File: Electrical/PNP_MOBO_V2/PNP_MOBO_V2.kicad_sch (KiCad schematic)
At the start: 48 parts, among them J1 USB_C_Receptacle_USB2.0_16P, J4 Conn_01x03_Pin, J6 Conn_01x03_Pin, J8 Barrel_Jack_MountingPin, SW1 SW_Push, SW2 SW_Push, U1 ESP32-S3-WROOM-1, U3 SN65HVD230, U4 AMS1117-3.3

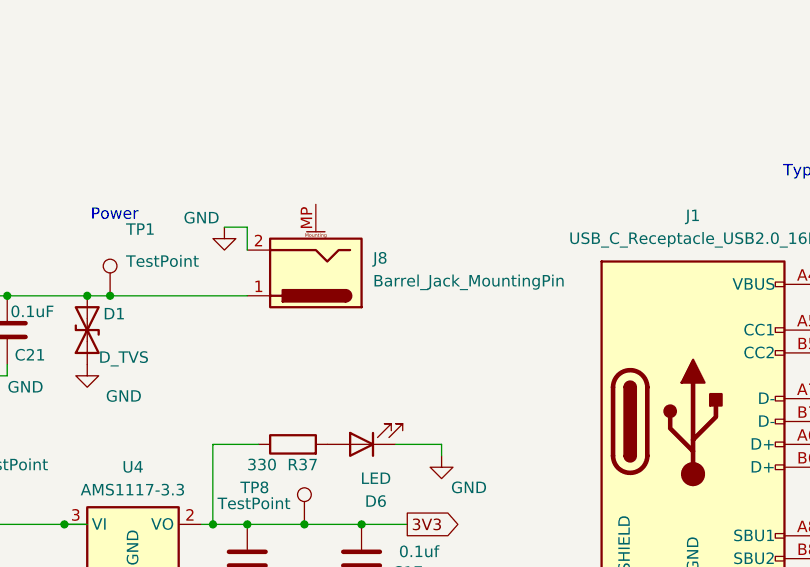
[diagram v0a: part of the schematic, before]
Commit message: fix: last change before order
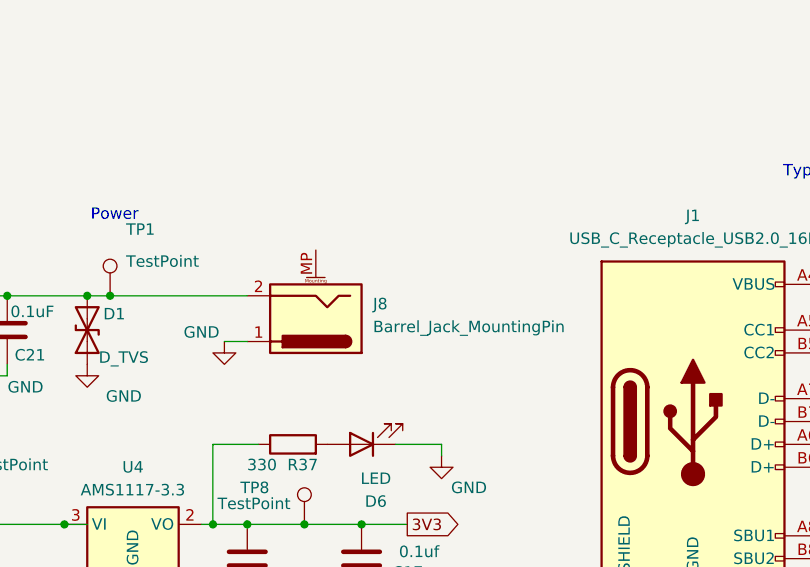
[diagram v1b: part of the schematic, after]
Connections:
- net 12V: now also J8.2; no longer J8.1
- net GND: now also J8.1; no longer J8.2
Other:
- moved on the sheet: J8
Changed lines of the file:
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@@
 	)
 	(junction
+		(at 39.37 151.13)
+		(diameter 0)
+		(color 0 0 0 0)
+	)
+	(junction
 		(at 60.96 184.15)
 		(diameter 0)
@@
 	)
 	(junction
-		(at 39.37 151.13)
-		(diameter 0)
-		(color 0 0 0 0)
-	)
-	(junction
 		(at 229.87 41.91)
 		(diameter 0)
@@
 	(wire
 		(pts
-			(xy 54.61 143.51) (xy 52.07 143.51)
+			(xy 54.61 156.21) (xy 52.07 156.21)
 		)
 		(stroke
@@
 	(wire
 		(pts
-			(xy 39.37 151.13) (xy 54.61 151.13)
-		)
-		(stroke
-			(width 0)
-			(type default)
-		)
-	)
-	(wire
-		(pts
 			(xy 27.94 160.02) (xy 25.4 160.02)
 		)
@@
 	(wire
 		(pts
-			(xy 54.61 146.05) (xy 54.61 143.51)
-		)
-		(stroke
-			(width 0)
-			(type default)
-		)
-	)
-	(wire
-		(pts
 			(xy 229.87 20.32) (xy 229.87 29.21)
 		)
@@
 	(wire
 		(pts
+			(xy 39.37 151.13) (xy 54.61 151.13)
+		)
+		(stroke
+			(width 0)
+			(type default)
+		)
+	)
+	(wire
+		(pts
 			(xy 134.62 167.64) (xy 148.59 167.64)
 		)
@@
 	(symbol
 		(lib_id "Connector:Barrel_Jack_MountingPin")
-		(at 62.23 148.59 180)
+		(at 62.23 153.67 180)
 		(unit 1)
 		(exclude_from_sim no)
@@
 		(fields_autoplaced yes)
 		(property "Reference" "J8"
-			(at 68.58 146.9643 0)
+			(at 68.58 152.0443 0)
 			(effects
 				(font
@@
 		)
 		(property "Value" "Barrel_Jack_MountingPin"
-			(at 68.58 149.5043 0)
+			(at 68.58 154.5843 0)
 			(effects
 				(font
@@
 		)
 		(property "Footprint" "Connector_BarrelJack:BarrelJack_CUI_PJ-063AH_Horizontal"
-			(at 60.96 147.574 0)
+			(at 60.96 152.654 0)
 			(effects
 				(font
@@
 		)
 		(property "Datasheet" "~"
-			(at 60.96 147.574 0)
+			(at 60.96 152.654 0)
 			(effects
 				(font
@@
 		)
 		(property "Description" "DC Barrel Jack with a mounting pin"
-			(at 62.23 148.59 0)
+			(at 62.23 153.67 0)
 			(effects
 				(font
@@
 	(symbol
 		(lib_id "power:GND")
-		(at 52.07 143.51 0)
+		(at 52.07 156.21 0)
 		(unit 1)
 		(exclude_from_sim no)
@@
 		(dnp no)
 		(property "Reference" "#PWR05"
-			(at 52.07 149.86 0)
+			(at 52.07 162.56 0)
 			(effects
 				(font
@@
 		)
 		(property "Value" "GND"
-			(at 49.53 142.494 0)
+			(at 49.53 155.194 0)
 			(effects
 				(font
@@
 		)
 		(property "Footprint" ""
-			(at 52.07 143.51 0)
+			(at 52.07 156.21 0)
 			(effects
 				(font
@@
 		)
 		(property "Datasheet" ""
-			(at 52.07 143.51 0)
+			(at 52.07 156.21 0)
 			(effects
 				(font
@@
 		)
 		(property "Description" "Power symbol creates a global label with name \"GND\" , ground"
-			(at 52.07 143.51 0)
+			(at 52.07 156.21 0)
 			(effects
 				(font
